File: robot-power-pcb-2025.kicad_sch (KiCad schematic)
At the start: 25 parts, among them J1 B14B-PHDSS, J10 B2B-PH, J11 B2B-PH, J12 B4B-PH, J13 B4B-PH, J2 XT60, J3 Conn_01x02, J4 Conn_01x02, J5 XT30, J6 XT30, J7 B2B-PH, J8 B2B-PH, J9 B2B-PH, K1 Relay_SPDT, U1 BigTreeTechV1.3_Module, U2 BigTreeTechV1.3_Module, U3 Sabertooth 2X5, U4 Sabertooth 2X5

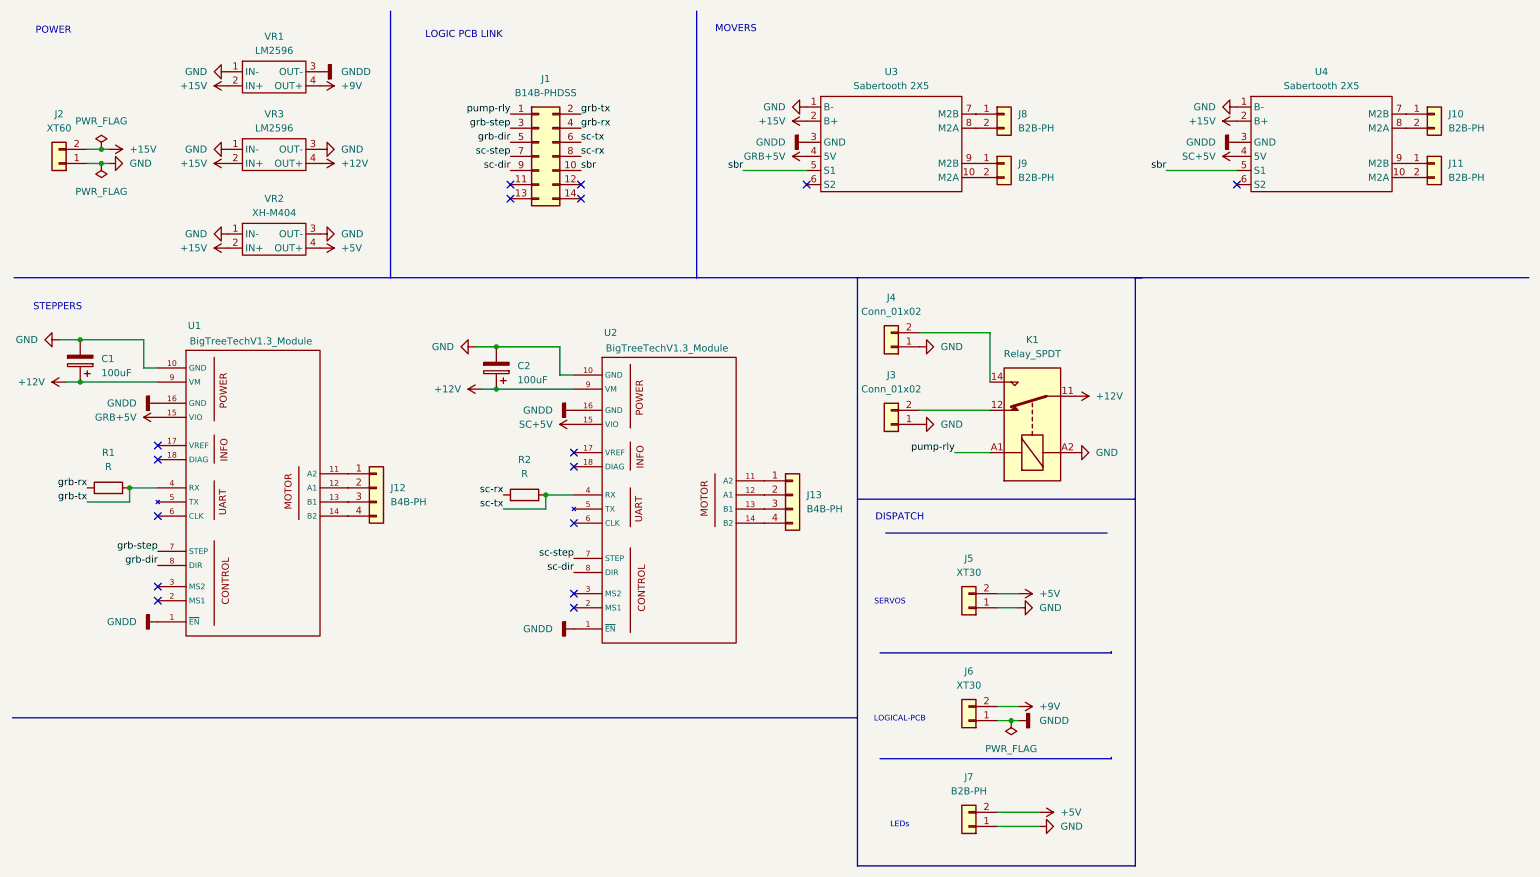
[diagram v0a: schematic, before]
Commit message: fix schematics
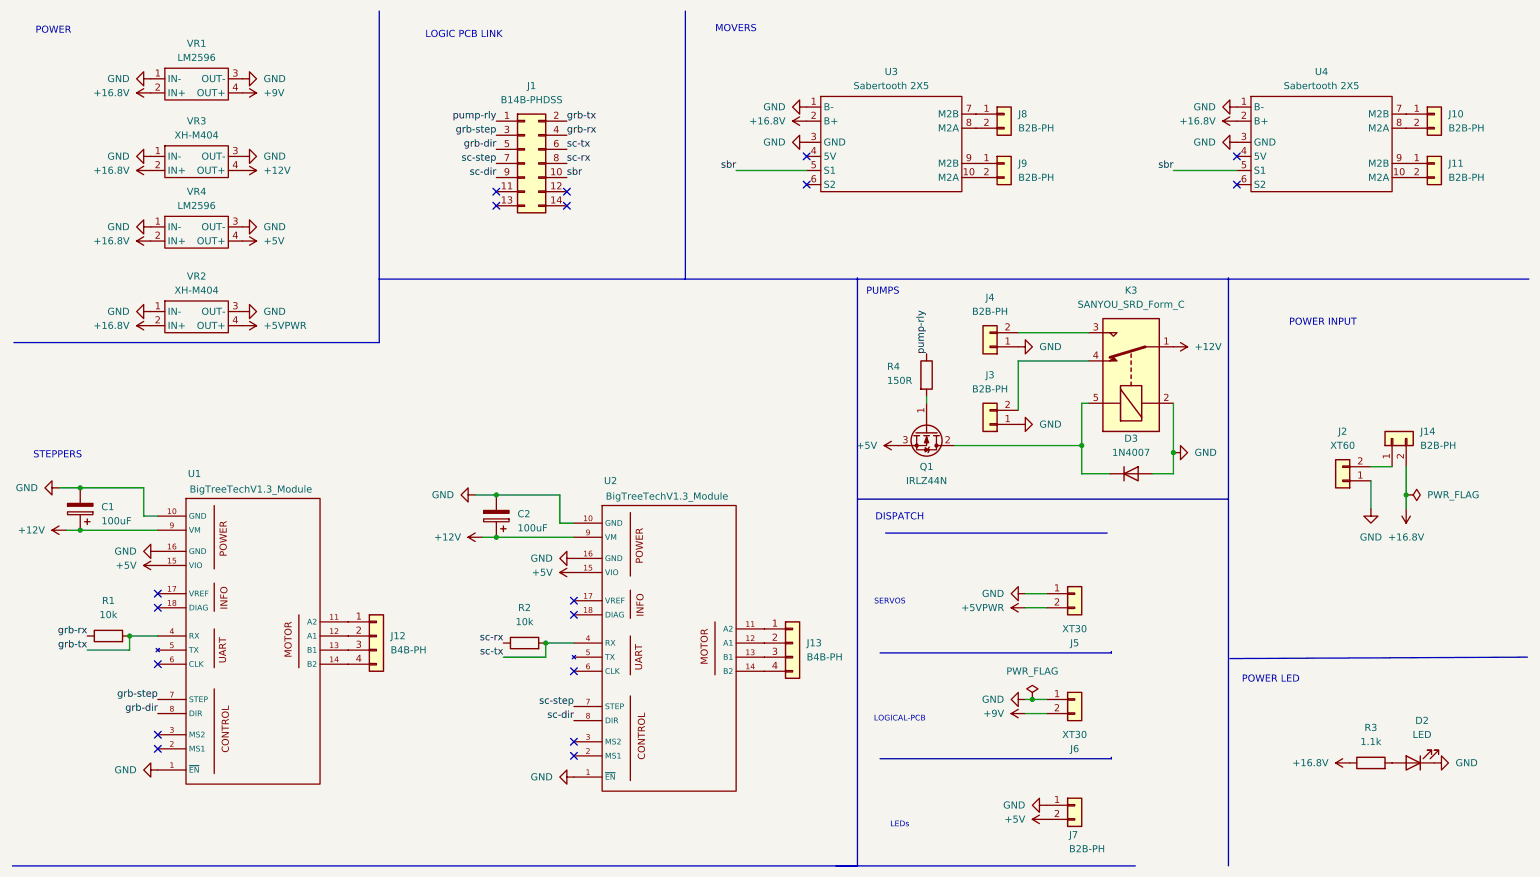
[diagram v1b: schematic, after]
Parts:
- removed K1: Relay_SPDT, symbol Relay:Relay_SPDT
- added D2: LED, LED_THT:LED_D5.0mm, symbol Device:LED
- added D3: 1N4007, Diode_THT:D_A-405_P7.62mm_Horizontal, symbol Device:D
- added J14: B2B-PH, Connector_JST:JST_PH_B2B-PH-K_1x02_P2.00mm_Vertical, symbol Connector_Generic:Conn_01x02
- added K3: SANYOU_SRD_Form_C, Relay_THT:Relay_SPDT_SANYOU_SRD_Series_Form_C, symbol Relay:SANYOU_SRD_Form_C
- added Q1: IRLZ44N, Package_TO_SOT_THT:TO-220-3_Horizontal_TabDown, symbol Transistor_FET:IRLZ44N
- added R3: 1.1k, Resistor_THT:R_Axial_DIN0207_L6.3mm_D2.5mm_P7.62mm_Horizontal, symbol Device:R
- added R4: 150R, Resistor_THT:R_Axial_DIN0207_L6.3mm_D2.5mm_P7.62mm_Horizontal, symbol Device:R
- added VR4: LM2596, Project:LM2596, symbol Project:Voltage_Regulator_Module
- C1, C2: footprint (none) -> Capacitor_THT:CP_Radial_D6.3mm_P2.50mm
- J10, J11, J7, J8, J9: footprint (none) -> Connector_JST:JST_PH_B2B-PH-K_1x02_P2.00mm_Vertical
- J12, J13: footprint (none) -> Connector_JST:JST_PH_B4B-PH-K_1x04_P2.00mm_Vertical
- J2: footprint (none) -> Connector_AMASS:AMASS_XT60-M_1x02_P7.20mm_Vertical
- J3, J4: value Conn_01x02 -> B2B-PH; footprint (none) -> Connector_JST:JST_PH_B2B-PH-K_1x02_P2.00mm_Vertical
- J5, J6: footprint (none) -> Connector_AMASS:AMASS_XT30UPB-M_1x02_P5.0mm_Vertical
- R1, R2: value R -> 10k; footprint (none) -> Resistor_THT:R_Axial_DIN0207_L6.3mm_D2.5mm_P7.62mm_Horizontal
- VR1: footprint (none) -> Project:LM2596
- VR2: footprint (none) -> Project:XHM404_Module
- VR3: value LM2596 -> XH-M404; footprint (none) -> Project:XHM404_Module
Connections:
- net GNDD is gone; now on net GND: J6.1 (Pin_1), U1.1 (~{EN}), U1.16 (GND), U2.1 (~{EN}), U2.16 (GND), U3.3 (GND), U4.3 (GND), VR1.3 (OUT-)
- net +12V: now also K3.1
- net +5V: now also U1.15 (VIO), U2.15 (VIO), Q1.3 (S), VR4.4 (OUT+); no longer J5.2 (Pin_2), VR2.4 (OUT+)
- net GND: now also D2.1 (K), D3.2 (A), K3.2, VR4.1 (IN-), VR4.3 (OUT-)
- net pump-rly: now also R4.1
- net at J3.2 (Pin_2): now also K3.4
- net at J4.2 (Pin_2): now also K3.3
- net +15V renamed +16.8V
- net +16.8V: now also J14.2 (Pin_2), R3.1, VR4.2 (IN+); no longer J2.2 (Pin_2)
- net GRB+5V: no longer names the net of U3.4 (5V)
- net GRB+5V: no longer U1.15 (VIO)
- net SC+5V: no longer names the net of U4.4 (5V)
- net SC+5V: no longer U2.15 (VIO)
- new net: J14.1 (Pin_1), J2.2 (Pin_2)
- new net: D2.2 (A), R3.2
- new net: D3.1 (K), K3.5, Q1.2 (D)
- new net: Q1.1 (G), R4.2
- new net +5VPWR: J5.2 (Pin_2), VR2.4 (OUT+)
- no-connect marks 16 -> 18
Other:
- note added: "POWER INPUT"
- note added: "POWER LED"
- note added: "PUMPS"
- moved on the sheet: C1, C2, J1, J12, J13, J3, J4, J5, J6, J7, R1, R2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
